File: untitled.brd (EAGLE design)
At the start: 100 x 80 mm, 7 parts

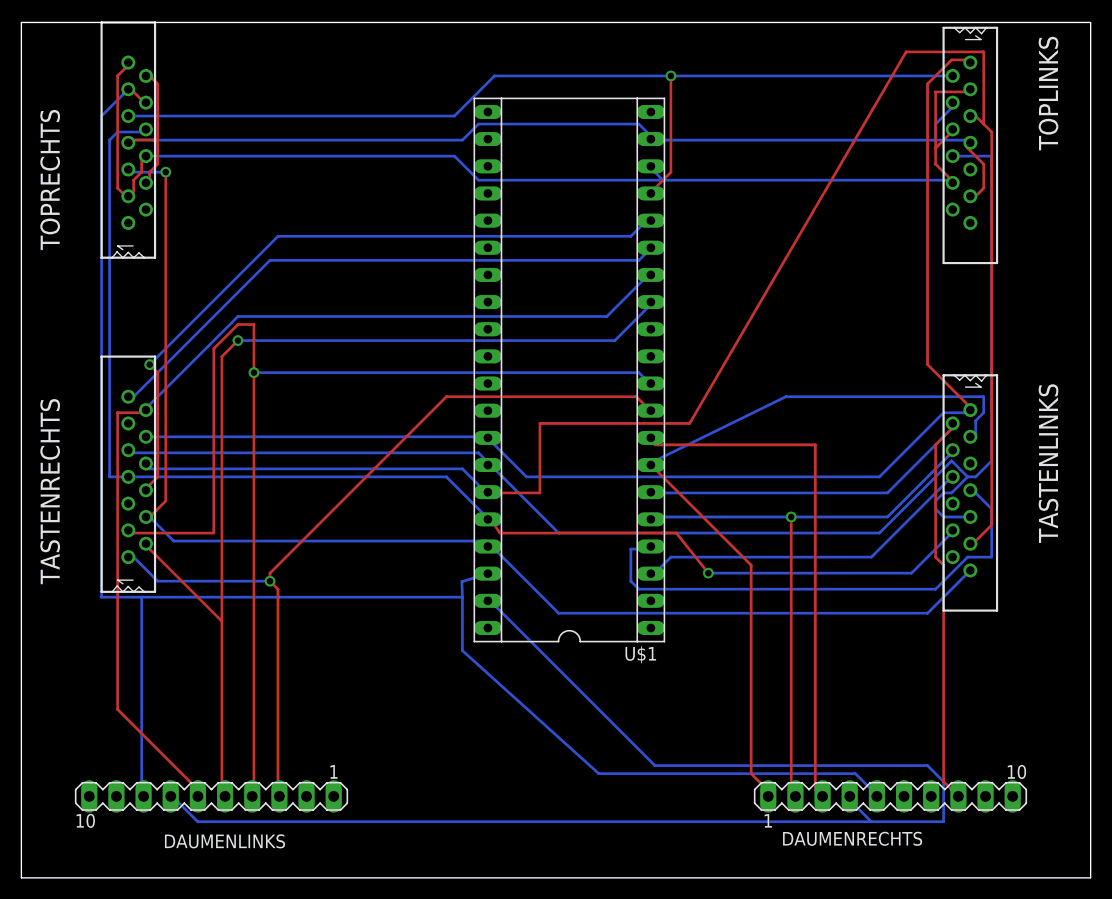
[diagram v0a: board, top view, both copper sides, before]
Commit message: board finished
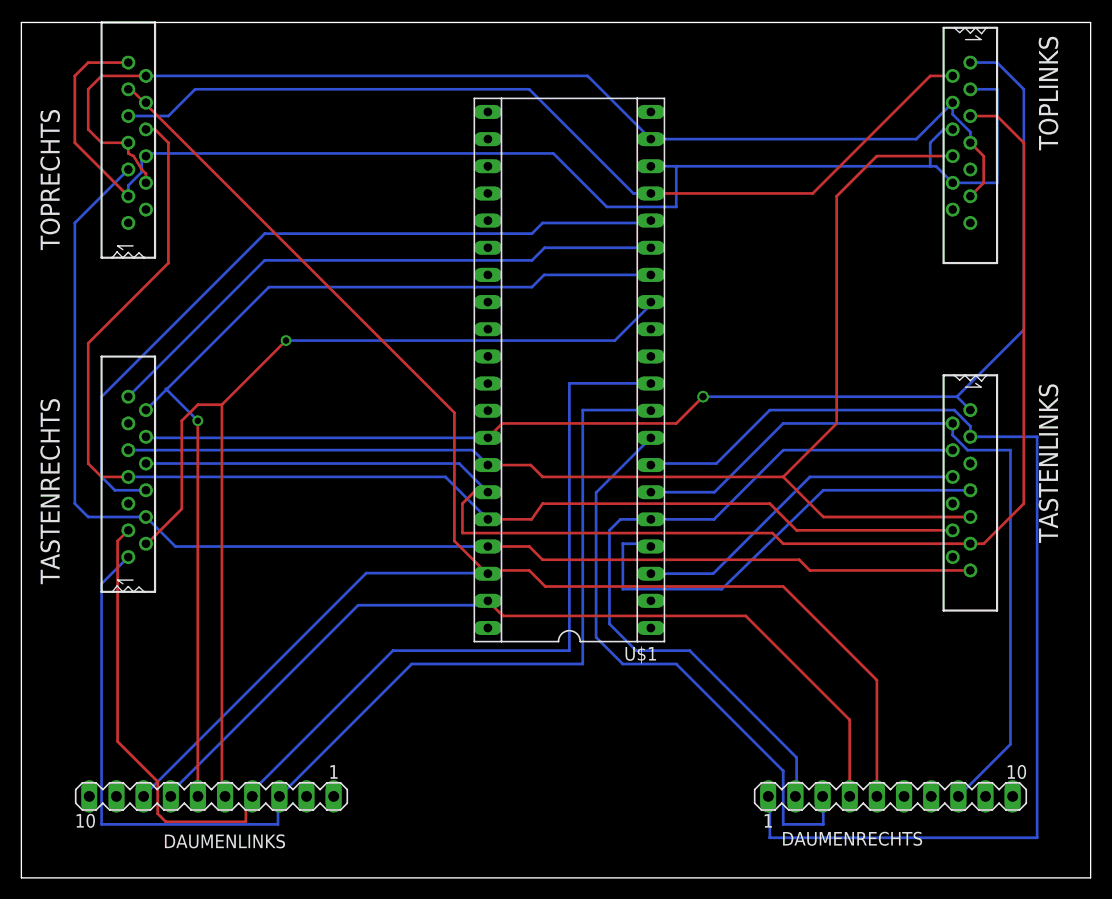
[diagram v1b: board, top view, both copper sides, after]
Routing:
- net B6: track 130.0 -> 83.1 mm
- net D4: track 72.8 -> 106.5 mm
- net D6: track 78.4 -> 109.1 mm, vias 1 -> 0
- net B2: track 155.1 -> 133.1 mm
- net C5: track 111.6 -> 127.9 mm
- net D2: track 57.2 -> 70.3 mm, vias 1 -> 0
- net B1: track 128.4 -> 122.1 mm
- net D5: track 48.9 -> 54.8 mm
- net C3: track 64.9 -> 70.4 mm, vias 1 -> 0
- net D3: track 67.5 -> 72.4 mm
- net C0: track 93.7 -> 98.2 mm
- net B5: track 156.1 -> 151.9 mm
- net C4: track 90.4 -> 86.7 mm, vias 1 -> 0
- net D1: track 47.4 -> 43.8 mm
- net D7: track 111.7 -> 108.2 mm, vias 1 -> 0
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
